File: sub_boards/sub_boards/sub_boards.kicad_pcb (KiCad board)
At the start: 2 copper layers, 84 x 105 mm, 18 parts, among them J1 Raspberry_Pi_5, J3 2.54mm PinHeader, J4 2.54mm PinHeader, Q1 ST-1KL3A, Q2 ST-1KL3A, Q3 ST-1KL3A, Q4 ST-1KL3A, SW1 TVBP06-B043CB-B, SW2 TVBP06-B043CB-B, SW3 TVBP06-B043CB-B, SW4 TVBP06-B043CB-B

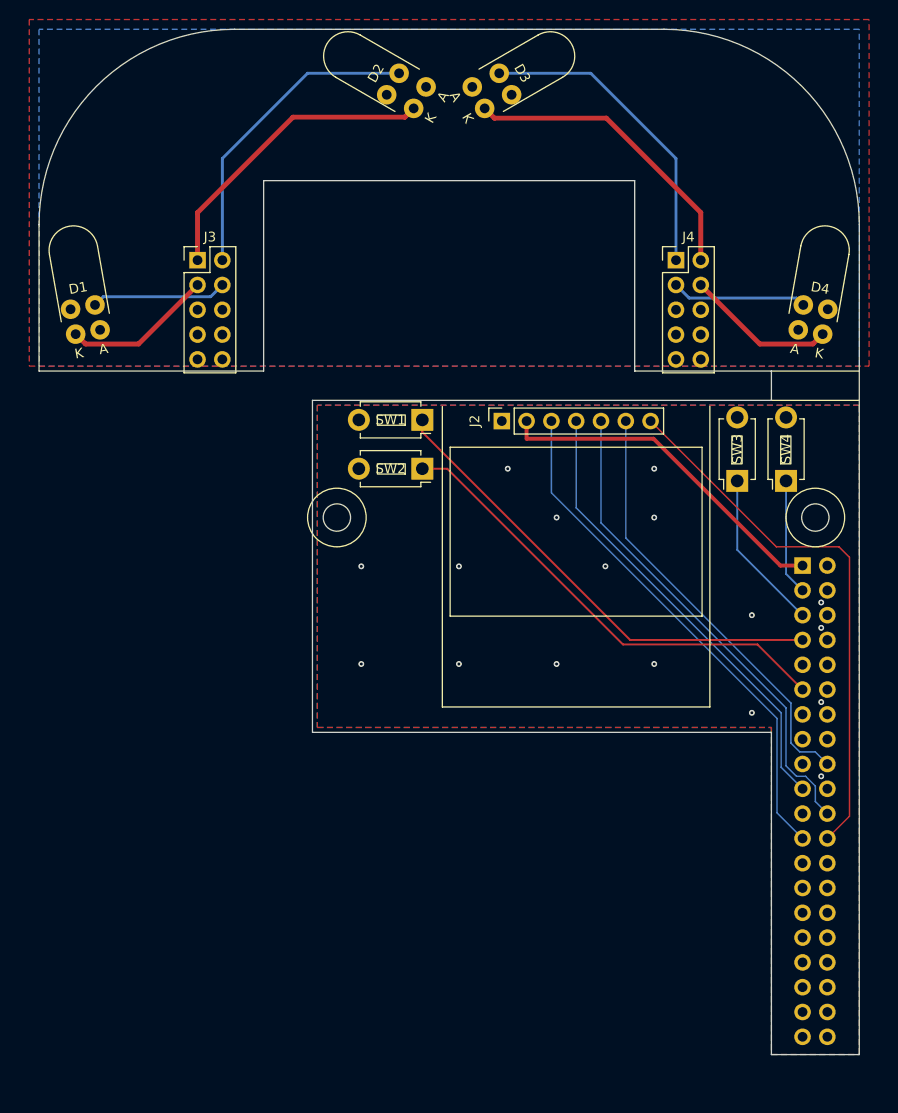
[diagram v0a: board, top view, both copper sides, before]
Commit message: 12/18 基板発注
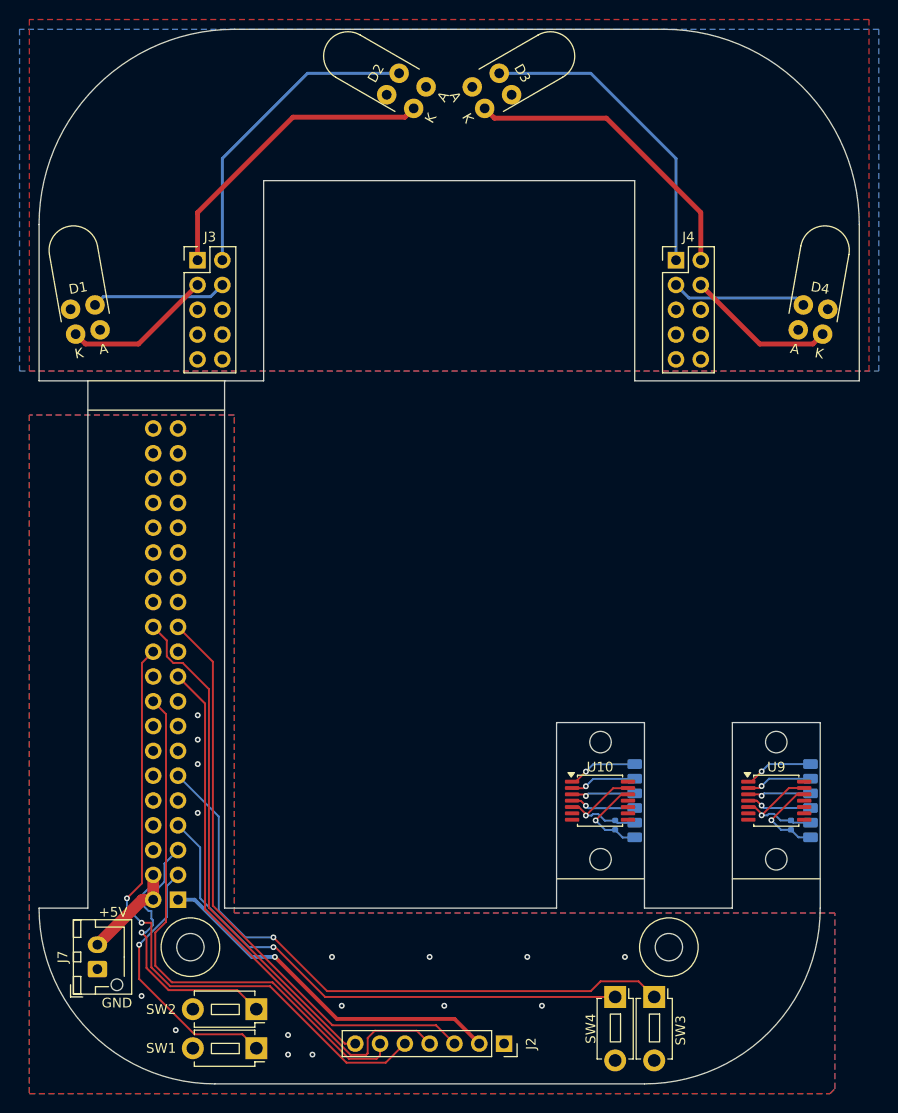
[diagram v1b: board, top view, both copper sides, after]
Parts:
- added C15: CC0603KRX7R9BB104, Capacitor_SMD:C_0402_1005Metric, B.Cu at (257.0, 116.5)
- added C16: CL05B104KO5NNNC, Capacitor_SMD:C_0402_1005Metric, B.Cu at (239.0, 116.5)
- added H3: M2 mounting hole, MountingHole:MountingHole_2.2mm_M2, F.Cu at (255.5, 120.0)
- added H4: M2 mounting hole, MountingHole:MountingHole_2.2mm_M2, F.Cu at (255.5, 108.0)
- added H5: M2 mounting hole, MountingHole:MountingHole_2.2mm_M2, F.Cu at (237.5, 120.0)
- added H6: M2 mounting hole, MountingHole:MountingHole_2.2mm_M2, F.Cu at (237.5, 108.0)
- added J5: EncSide, Library:EncoderPad, B.Cu at (259.0, 114.0)
- added J6: EncSide, Library:EncoderPad, B.Cu at (241.0, 114.0)
- added J7: B2B-XH, Connector_JST:JST_XH_B2B-XH-AM_1x02_P2.50mm_Vertical, F.Cu at (186.0, 131.2)
- added U10: AS5047D, Package_SO:TSSOP-14_4.4x5mm_P0.65mm, F.Cu at (237.4, 114.0)
- added U9: AS5047D, Package_SO:TSSOP-14_4.4x5mm_P0.65mm, F.Cu at (255.5, 114.0)
- moved H2 77.7 mm to (195.5, 129.0)
- moved J1 72.5 mm to (194.2, 124.1), turned to 0 degrees
- moved SW1 66.6 mm to (202.2, 139.4)
- moved J2 63.8 mm to (227.6, 138.9), turned to -90 degrees
- moved SW2 57.9 mm to (202.2, 135.4)
- moved SW4 55.7 mm to (239.0, 134.1), turned to -90 degrees
- moved H1 55.6 mm to (244.5, 129.0)
- moved SW3 53.5 mm to (243.0, 134.1), turned to -90 degrees
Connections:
- J1 pad 11: /BTN_UP -> /BTN_RIGHT
- J1 pad 2: unconnected-(J1-5V-Pad2) -> /+5V
- J1 pad 3: /BTN_LEFT -> /BTN_DOWN
- J1 pad 4: unconnected-(J1-5V-Pad4) -> /+5V
- J1 pad 5: /BTN_RIGHT -> /BTN_UP
- J1 pad 7: /BTN_DOWN -> /BTN_LEFT
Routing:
- net /BTN_RIGHT: track 16.5 -> 64.6 mm, vias 0 -> 1
- net /BTN_LEFT: track 11.9 -> 55.1 mm, vias 0 -> 1
- net /BTN_DOWN: track 49.0 -> 27.2 mm, vias 0 -> 1
- net /BTN_UP: track 48.3 -> 28.7 mm, vias 0 -> 1
- net /RES: track 50.3 -> 65.9 mm, vias 0 -> 2
- net Net-(J5-Pin_2): track 0.00 -> 12.8 mm, vias 0 -> 1
- net Net-(J6-Pin_2): track 0.00 -> 12.8 mm, vias 0 -> 1
- net /DC: track 44.6 -> 56.4 mm
- net /+5V: track 0.00 -> 10.2 mm
- net /MOSI: track 47.3 -> 56.7 mm
- net Net-(J5-Pin_1): track 0.00 -> 9.20 mm, vias 0 -> 1
- net Net-(J6-Pin_1): track 0.00 -> 9.20 mm, vias 0 -> 1
- net /SCLK: track 53.4 -> 60.6 mm
- net Net-(J6-Pin_6): track 0.00 -> 7.11 mm, vias 0 -> 1
- net Net-(J5-Pin_6): track 0.00 -> 7.11 mm, vias 0 -> 1
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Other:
- board size 84 x 105 mm -> 84 x 108 mm
- board text added: "+5V"
- board text added: "GND"
